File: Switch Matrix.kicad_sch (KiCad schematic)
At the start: 259 parts, among them SW1 SD_6B1D, SW10 SD_4B1E, SW100 SD_4B3E, SW101 SD_4B3E, SW102 SD_4B3E, SW103 SD_4B3E, SW104 SD_4B3E, SW105 SD_4B3E, SW106 SD_4B3E, SW107 SD_4B3E, SW108 SD_4B3E, SW109 SD_4B3E, SW11 SD_4B1E, SW110 SD_4B3E, SW111 SD_4B3E, SW112 SD_6B1D, SW113 SD_4B3E, SW114 SD_4B3E, SW115 UNPOPULATED, SW116 SD_4B3E, SW117 SD_5B3E, SW118 SD_4B3E, SW119 UNPOPULATED, SW12 SD_6B1D, SW120 SD_4B3E, SW121 SD_4B3E, SW122 SD_4B3E, SW122a0 UNPOPULATED, SW123 SD_4B3E, SW123a0 UNPOPULATED, SW124 UNPOPULATED, SW124a0 SD_4B3E, SW125 SD_4B3E, SW126 SD_4B3E, SW127 UNPOPULATED, SW128 SD_4B3E, SW13 SD_4B1E, SW14 SD_6B1D, SW15 SD_4B1E, SW16 SD_6B1D, SW17 SD_4B1E, SW18 SD_6B1D, SW19 SD_4B1E, SW2 SD_4B1E, SW20 SD_6B1D, SW21 SD_4B1E, SW22 SD_6B1D, SW23 SD_4B1E, SW24 SD_6B1D, SW25 SD_4B3E, SW26 SD_4B3E, SW27 SD_6B1D, SW28 SD_4B3E, SW29 SD_4B3E, SW3 SD_6B1D, SW30 SD_4B3E, SW31 SD_4B3E, SW32 SD_4B3E, SW33 SD_4B3E, SW34 SD_4B3E, SW35 SD_4B3E, SW36 SD_4B3E, SW37 SD_4B3E, SW38 SD_4B3E, SW39 SD_4B3E, SW4 SD_4B1E, SW40 SD_4B3E, SW41 UNPOPULATED, SW42 SD_4B3E, SW43 SD_4B3E, SW44 SD_4B3E, SW45 SD_4B3E, SW46 SD_6B1D, SW47 SD_4B3E, SW48 SD_4B3E, SW49 SD_4B3E, SW5 SD_6B1D, SW50 SD_4B3E, SW51 SD_4B3E, SW52 SD_6B1D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

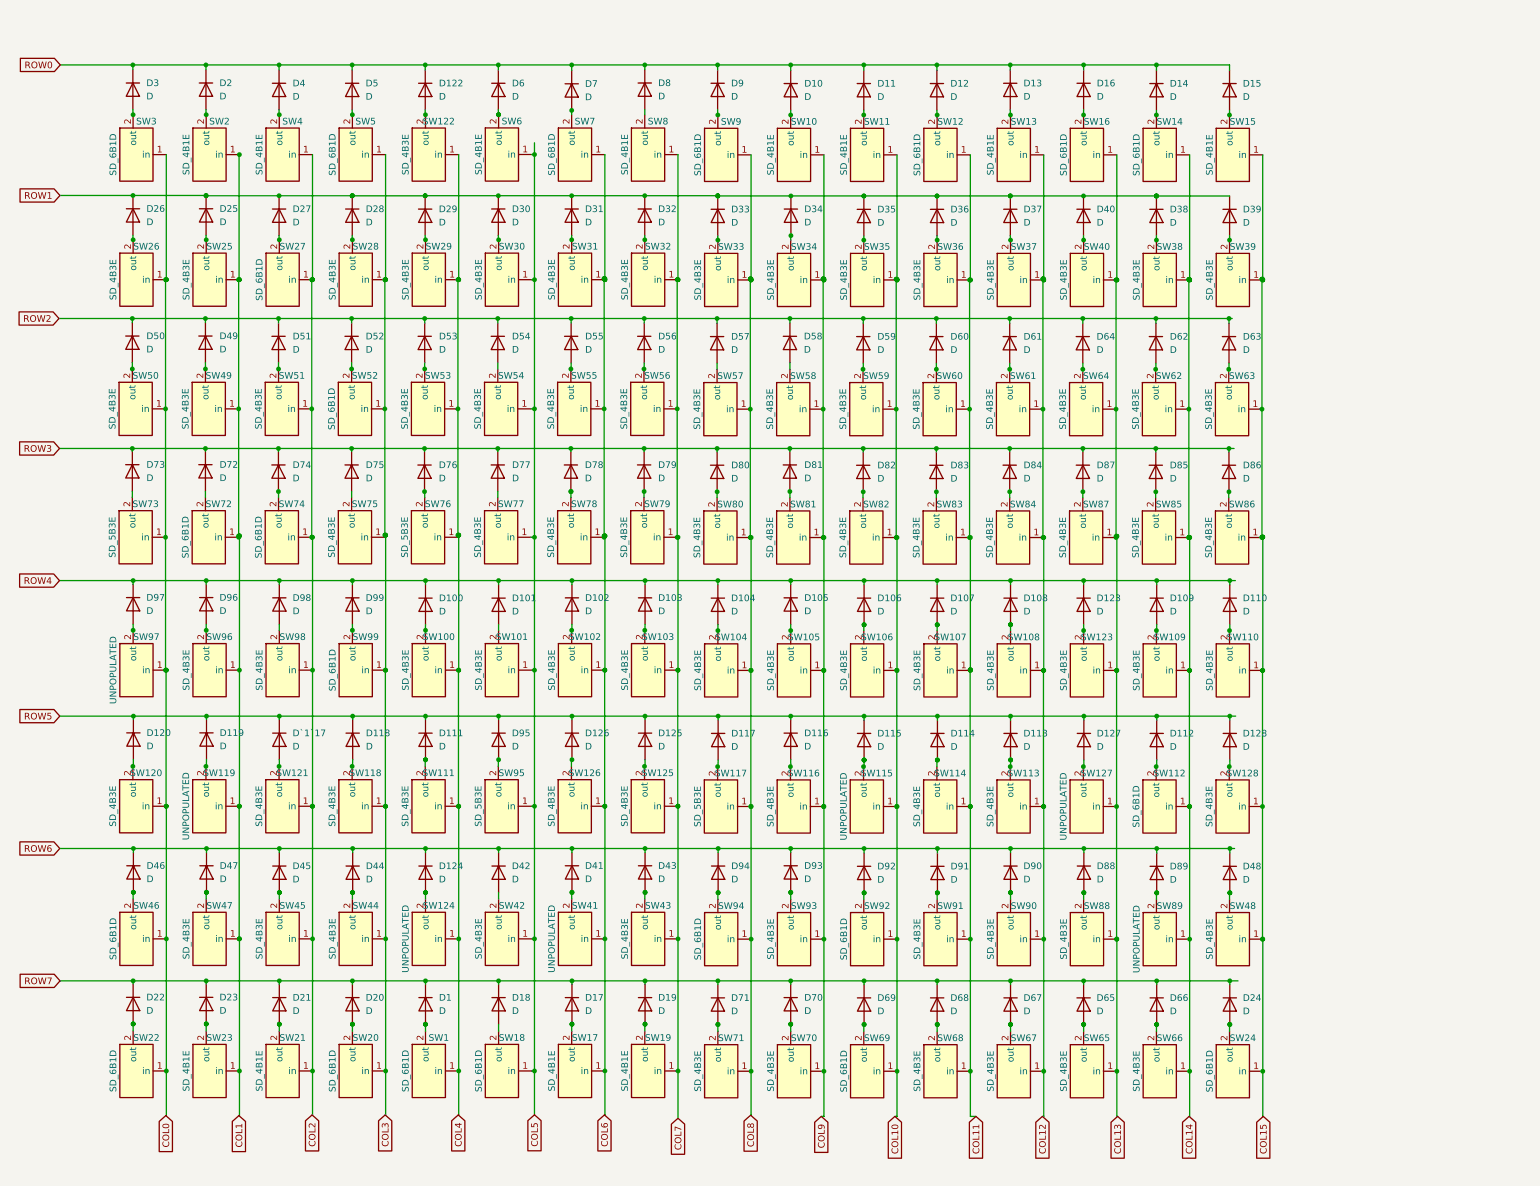
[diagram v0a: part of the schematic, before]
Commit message: wip: big matrix fix and starting routing
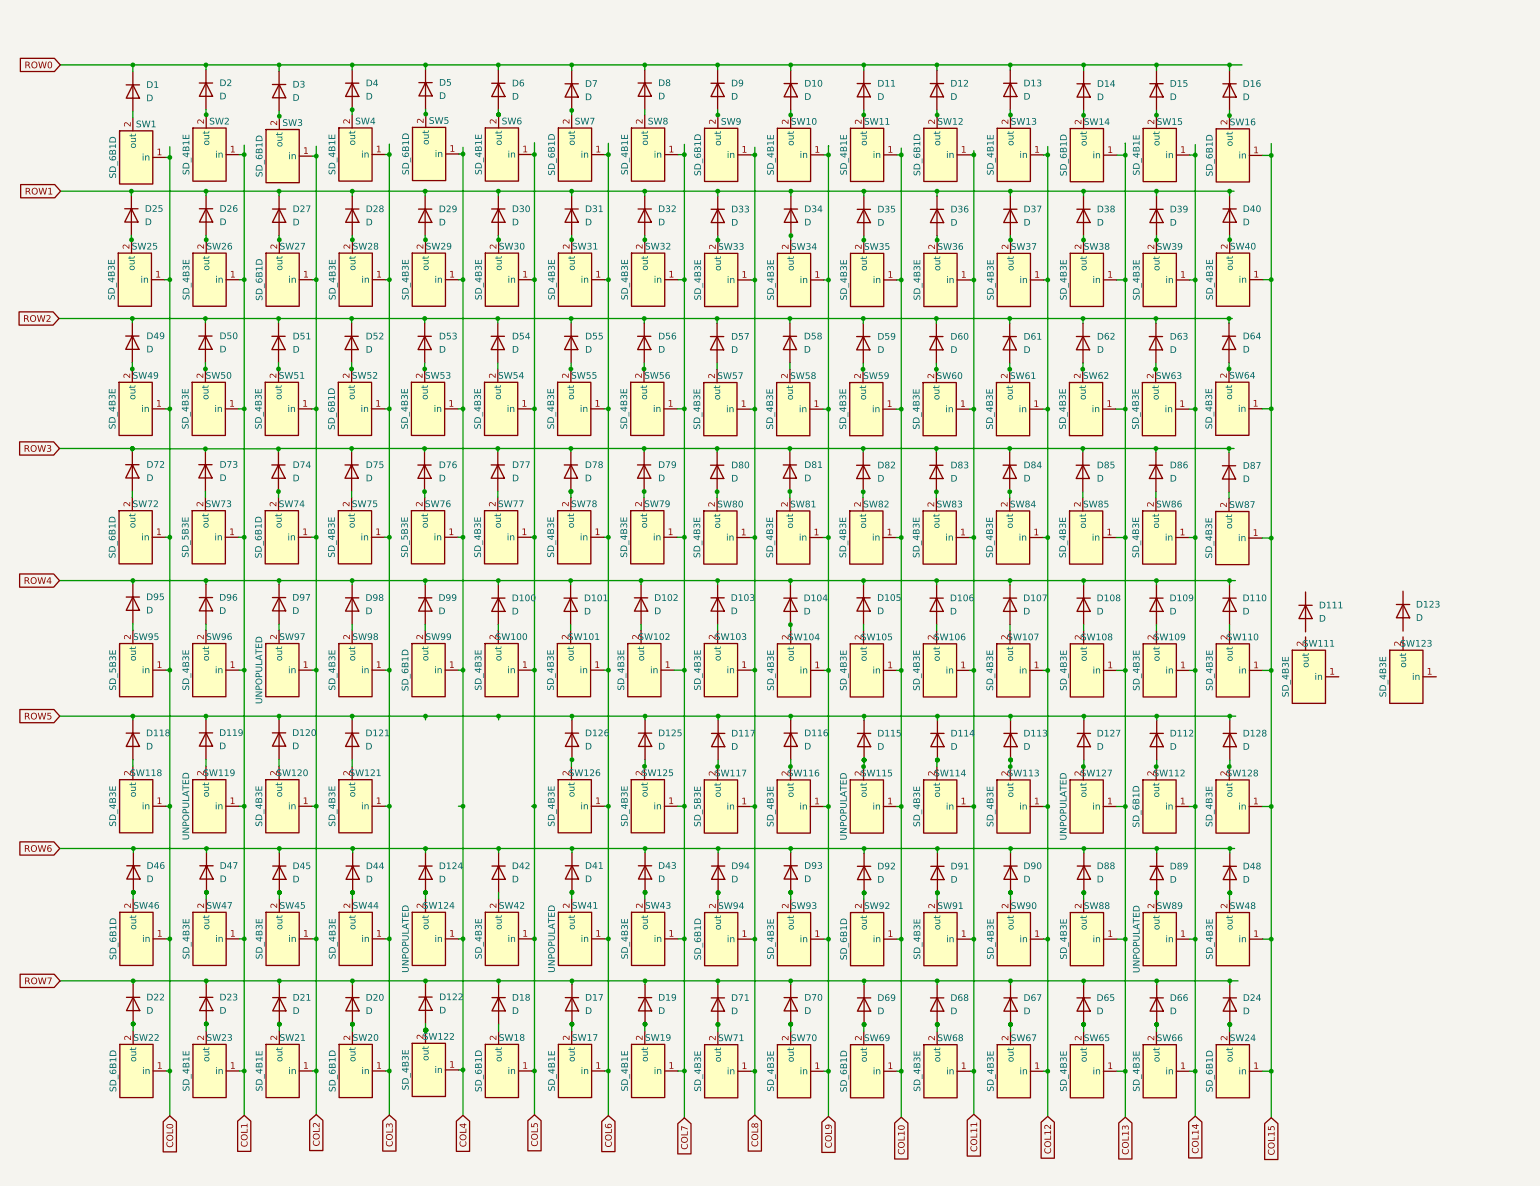
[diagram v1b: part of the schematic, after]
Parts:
- renumbered D`1`17 to D121
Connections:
- net COL0: now also SW1.1 (in), SW118.1 (in), SW25.1 (in), SW49.1 (in), SW72.1 (in), SW95.1 (in); no longer SW120.1 (in), SW26.1 (in), SW3.1 (in), SW50.1 (in), SW73.1 (in), SW97.1 (in)
- net COL1: now also SW26.1 (in), SW50.1 (in), SW73.1 (in); no longer SW25.1 (in), SW49.1 (in), SW72.1 (in)
- net COL10: now also SW105.1 (in); no longer SW106.1 (in)
- net COL11: now also SW106.1 (in); no longer SW107.1 (in)
- net COL12: now also SW107.1 (in); no longer SW108.1 (in)
- net COL13: now also SW108.1 (in), SW14.1 (in), SW38.1 (in), SW62.1 (in), SW85.1 (in); no longer SW123.1 (in), SW16.1 (in), SW40.1 (in), SW64.1 (in), SW87.1 (in)
- net COL14: now also SW15.1 (in), SW39.1 (in), SW63.1 (in), SW86.1 (in); no longer SW14.1 (in), SW38.1 (in), SW62.1 (in), SW85.1 (in)
- net COL15: now also SW16.1 (in), SW40.1 (in), SW64.1 (in), SW87.1 (in); no longer SW15.1 (in), SW39.1 (in), SW63.1 (in), SW86.1 (in)
- net COL2: now also SW120.1 (in), SW3.1 (in), SW97.1 (in); no longer SW121.1 (in), SW4.1 (in), SW98.1 (in)
- net COL3: now also SW121.1 (in), SW4.1 (in), SW98.1 (in); no longer SW118.1 (in), SW5.1 (in), SW99.1 (in)
- net COL4: now also SW5.1 (in), SW99.1 (in); no longer SW1.1 (in), SW100.1 (in), SW111.1 (in)
- net COL5: now also SW100.1 (in); no longer SW101.1 (in), SW95.1 (in)
- net COL6: now also SW101.1 (in); no longer SW102.1 (in)
- net COL7: now also SW102.1 (in); no longer SW103.1 (in)
- net COL8: now also SW103.1 (in); no longer SW104.1 (in)
- net COL9: now also SW104.1 (in); no longer SW105.1 (in)
- net ROW0: now also D1.1 (K); no longer D122.1 (K)
- net ROW4: now also D95.1 (K); no longer D123.1 (K)
- net ROW5: no longer D111.1 (K), D95.1 (K)
- net ROW7: now also D122.1 (K); no longer D1.1 (K)
- net at SW123.2 (out): no longer D123.2 (A)
- net at D111.2 (A): no longer SW111.2 (out)
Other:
- moved on the sheet: D1, D100, D101, D102, D103, D104, D105, D106, D107, D108, D111, D118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

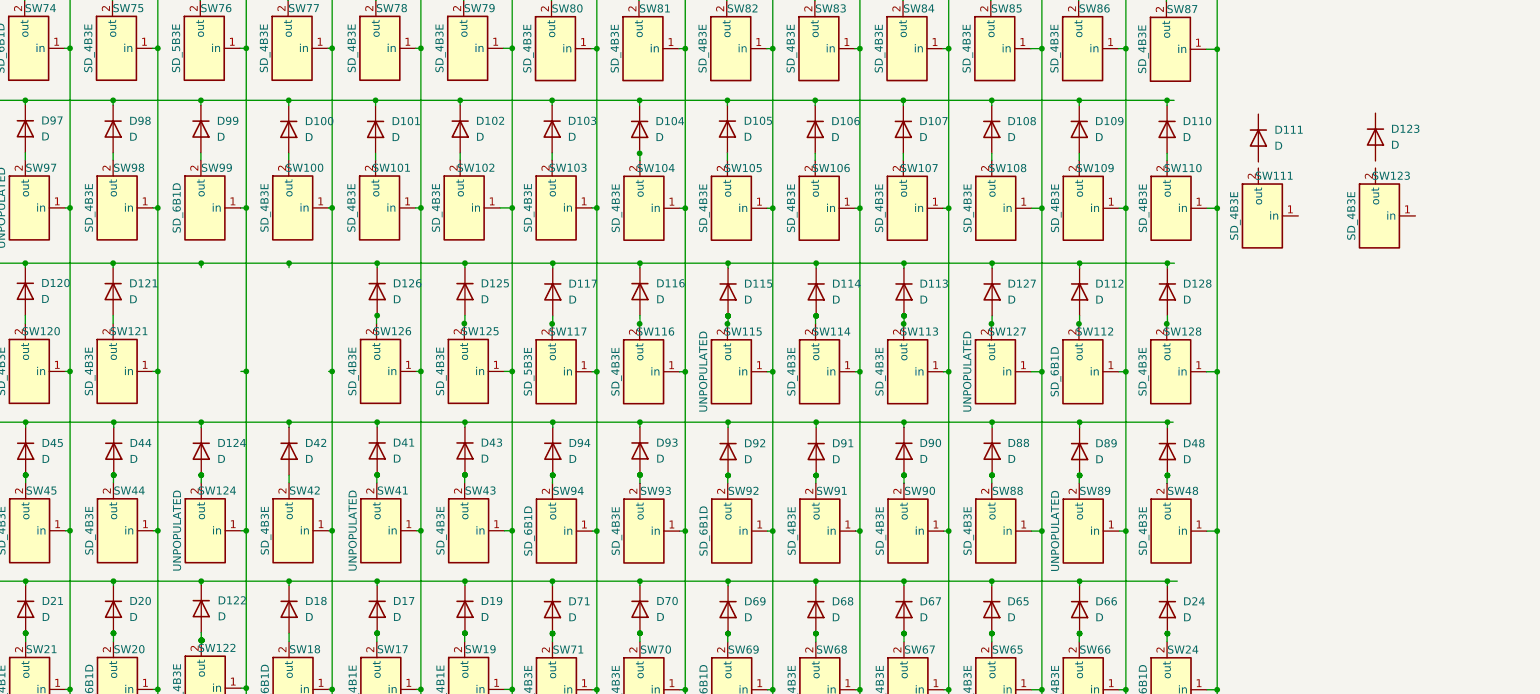
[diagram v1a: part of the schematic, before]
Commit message: wip: small matrix fix and continue routing
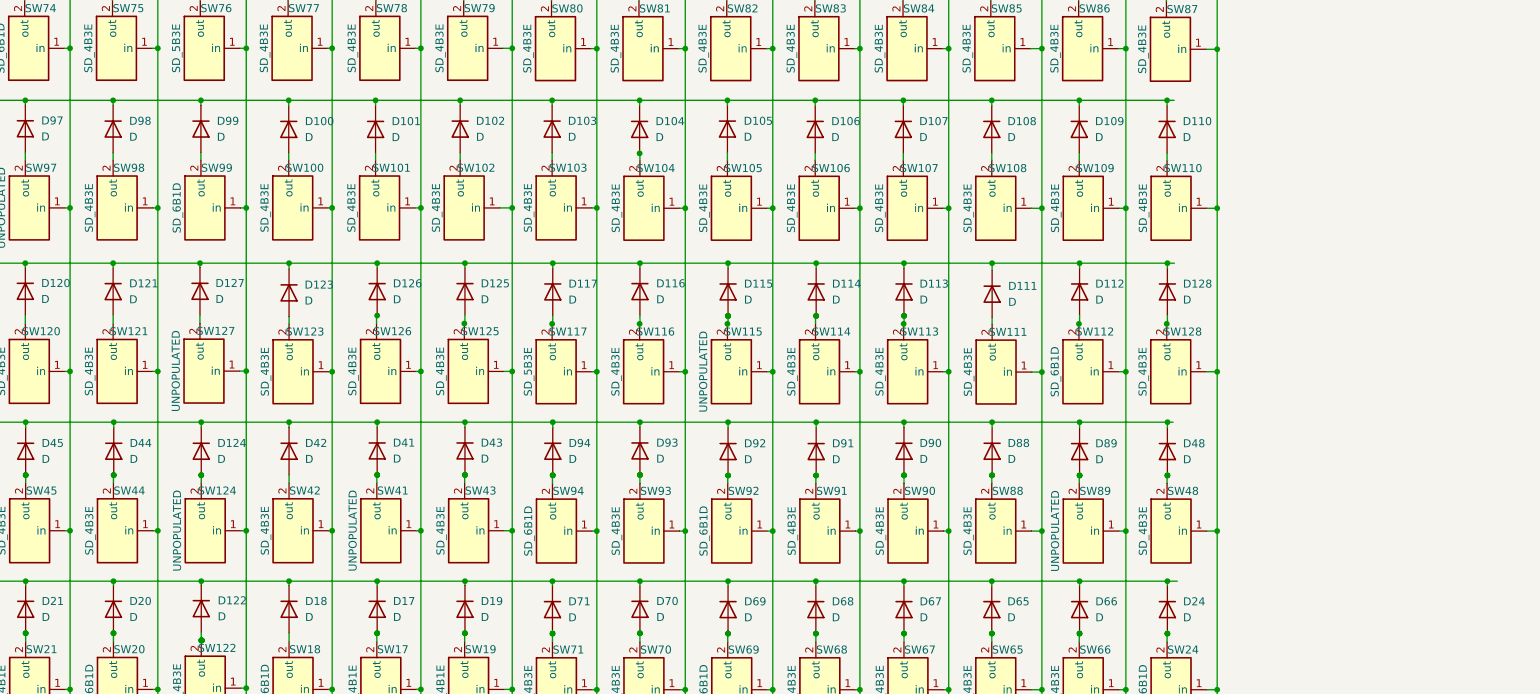
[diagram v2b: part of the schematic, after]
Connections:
- net COL13: now also SW111.1 (in); no longer SW127.1 (in)
- net COL4: now also SW127.1 (in)
- net COL5: now also SW123.1 (in)
- net ROW5: now also D111.1 (K), D123.1 (K)
- net at SW123.2 (out): now also D123.2 (A)
- net at D111.2 (A): now also SW111.2 (out)
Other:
- moved on the sheet: D111, D123, D127, SW111, SW123, SW127
